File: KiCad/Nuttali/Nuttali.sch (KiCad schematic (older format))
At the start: 0 parts

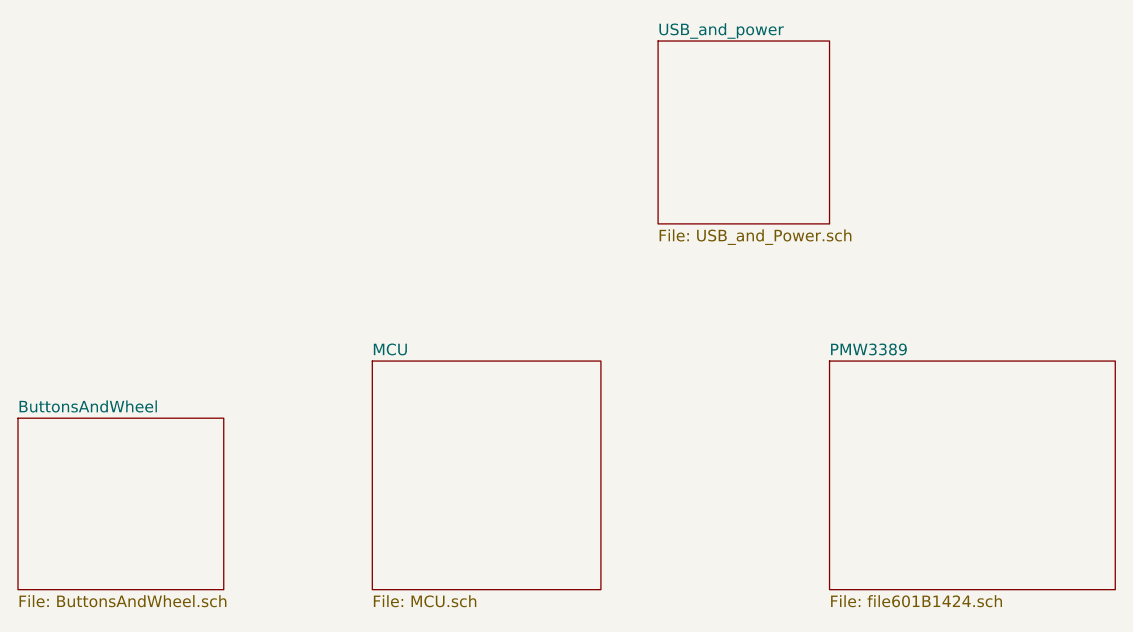
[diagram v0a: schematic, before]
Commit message: some footprints fixed
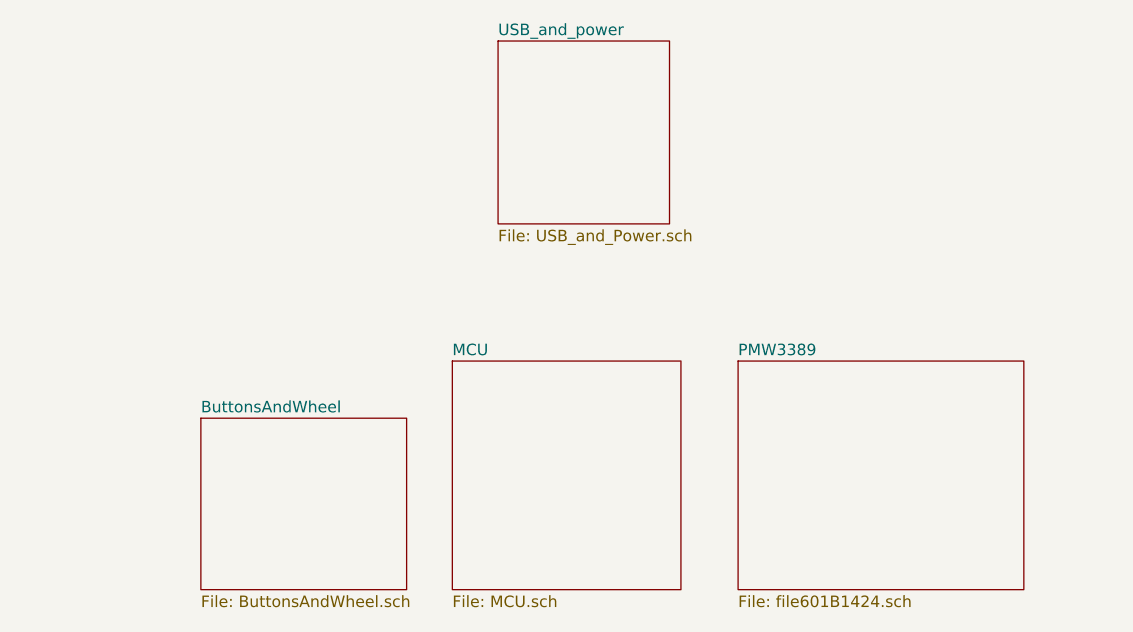
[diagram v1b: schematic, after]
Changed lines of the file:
@@
 $EndDescr
 $Sheet
-S 5000 2500 1000 1000
+S 5350 2500 1000 1000
 U 6022F0F9
 F0 "MCU" 50
@@
 $EndSheet
 $Sheet
-S 7000 2500 1250 1000
+S 6600 2500 1250 1000
 U 601B1425
 F0 "PMW3389" 50
@@
 $EndSheet
 $Sheet
-S 6250 1100 750  800
+S 5550 1100 750  800
 U 601D470C
 F0 "USB_and_power" 50
@@
 $EndSheet
 $Sheet
-S 3450 2750 900  750
+S 4250 2750 900  750
 U 6022DC9B
 F0 "ButtonsAndWheel" 50

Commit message: First draft of the pcb
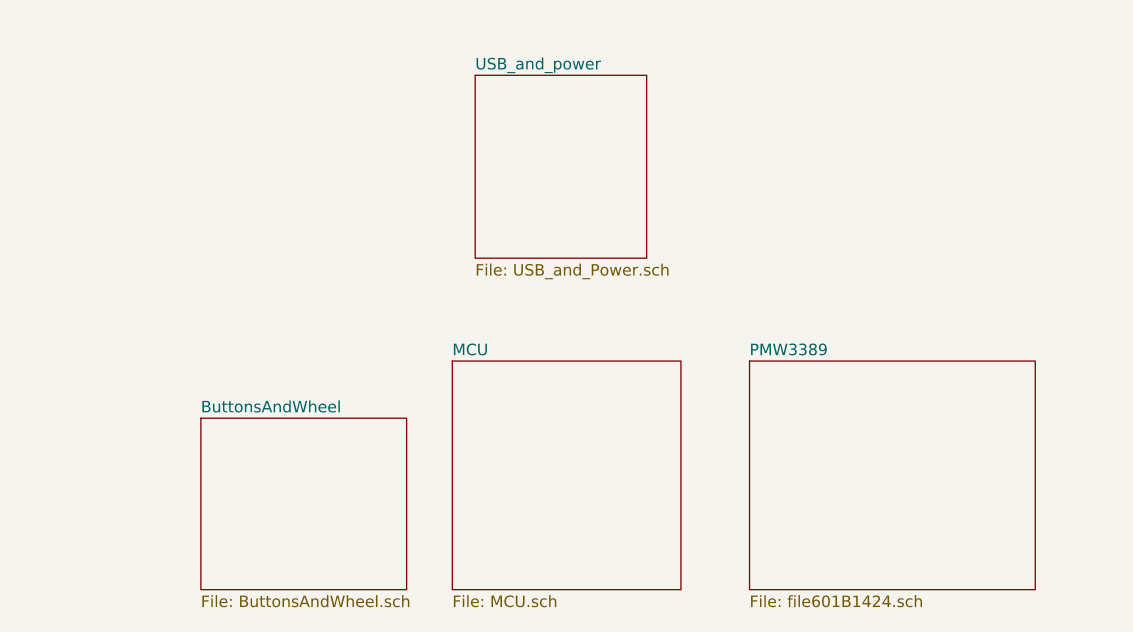
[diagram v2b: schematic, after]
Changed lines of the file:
@@
 $EndSheet
 $Sheet
-S 6600 2500 1250 1000
+S 6650 2500 1250 1000
 U 601B1425
 F0 "PMW3389" 50
@@
 $EndSheet
 $Sheet
-S 5550 1100 750  800
+S 5450 1250 750  800
 U 601D470C
 F0 "USB_and_power" 50
